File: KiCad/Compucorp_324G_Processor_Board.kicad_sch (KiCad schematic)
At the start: 9 parts, among them J5 Processor Interboard, J6 Test Connector, U5 TMC1872 (TCL07), U6 TMC1866 (TCL06), U7 TMC1867 (TCL05), U8 TMC1870 (TCL04)

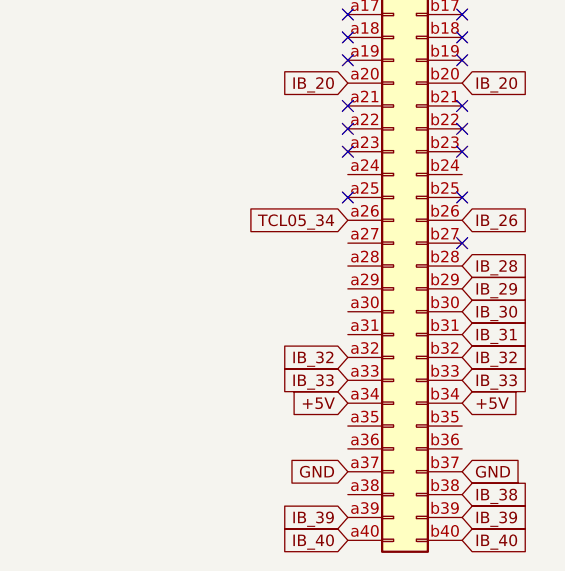
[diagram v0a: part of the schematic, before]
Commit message: Update Compucorp_324G_Processor_Board.kicad_sch
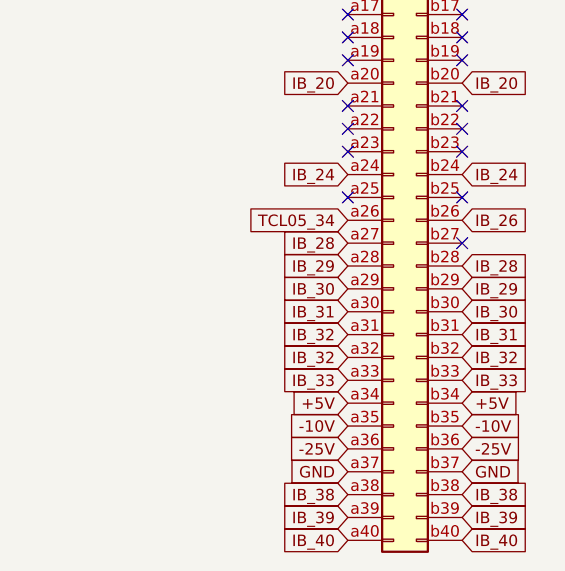
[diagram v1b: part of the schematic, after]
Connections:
- net IB_28: now also J5.a27 (Pin_a27)
- net IB_29: now also J5.a28 (Pin_a28)
- net IB_30: now also J5.a29 (Pin_a29)
- net IB_31: now also J5.a30 (Pin_a30)
- net IB_32: now also J5.a31 (Pin_a31)
- net IB_38: now also J5.a38 (Pin_a38)
- net IB_24: now reaches J5.a24 (Pin_a24)
- net IB_24: now also J5.b24 (Pin_b24)
- net -10V: now reaches J5.a35 (Pin_a35)
- net -10V: now also J5.b35 (Pin_b35)
- net -25V: now reaches J5.a36 (Pin_a36)
- net -25V: now also J5.b36 (Pin_b36)

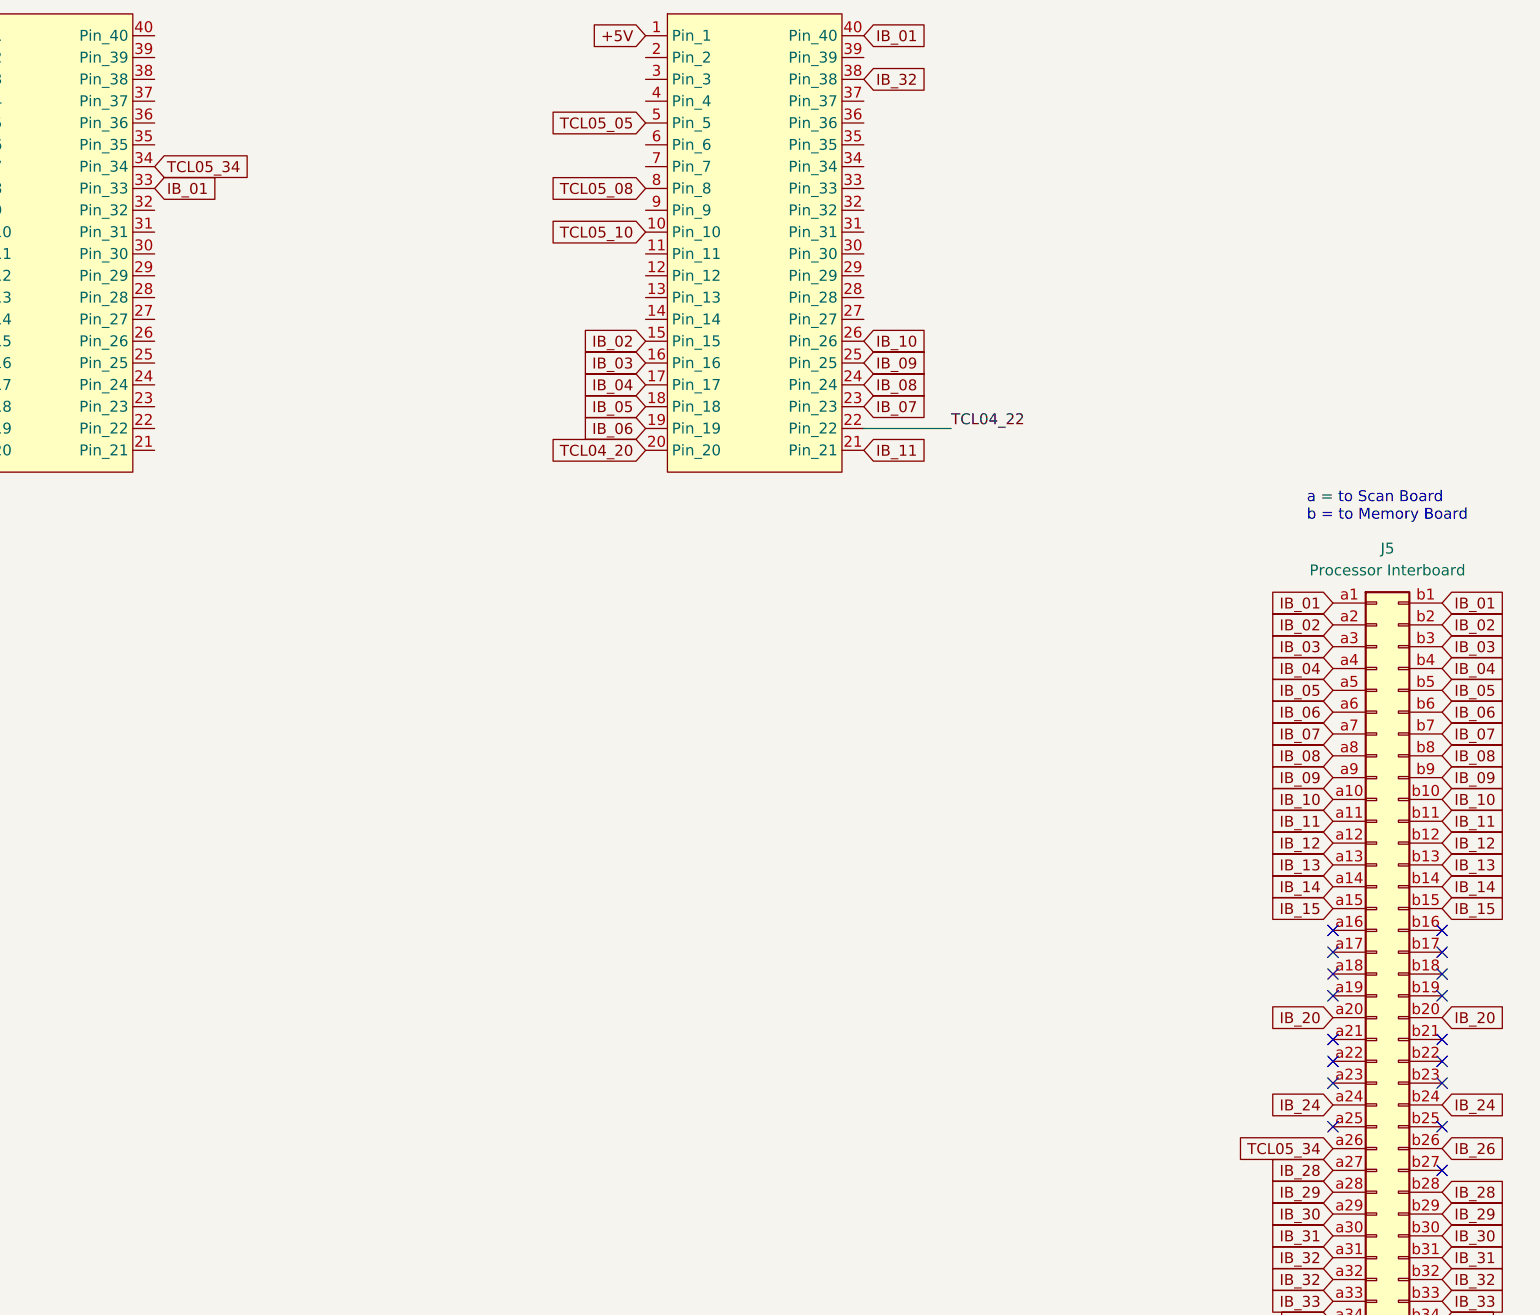
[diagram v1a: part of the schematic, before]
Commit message: Update Compucorp_324G_Processor_Board.kicad_sch
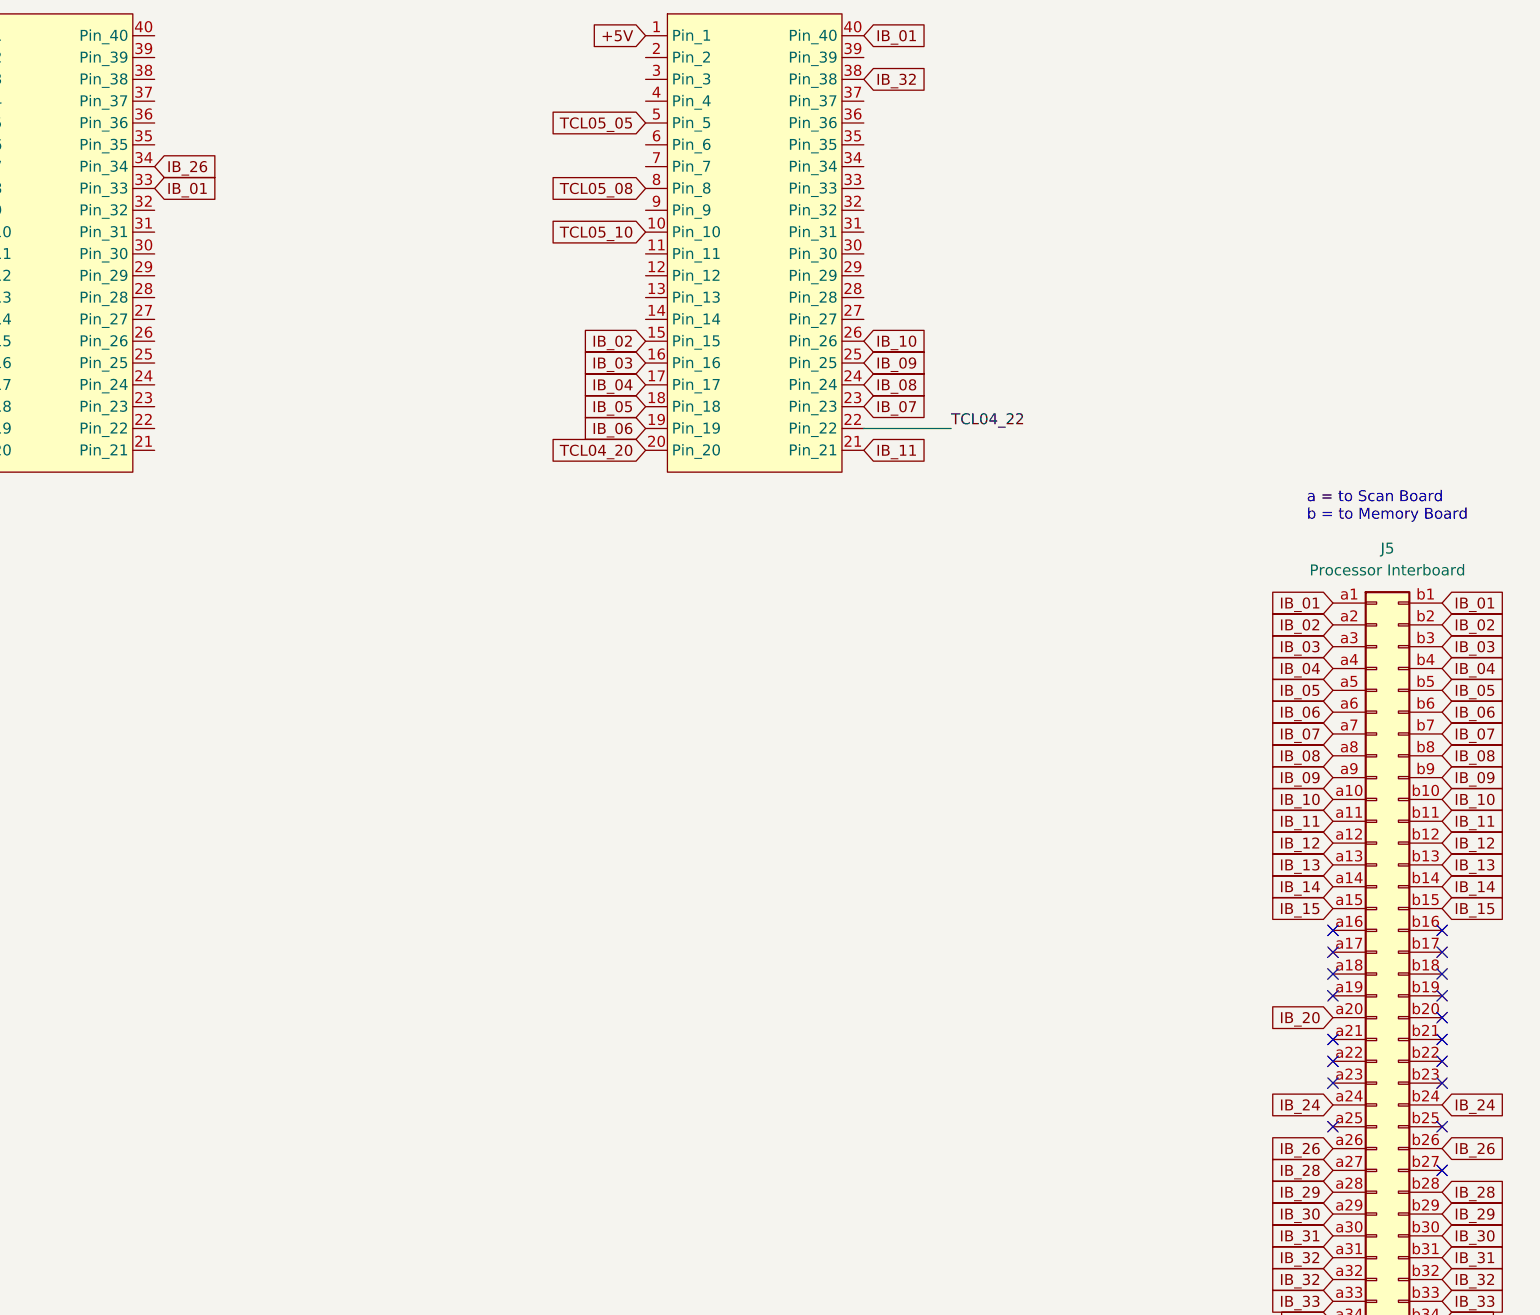
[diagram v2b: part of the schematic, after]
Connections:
- net TCL05_34 is gone; now on net IB_26: J5.a26 (Pin_a26), U7.34 (Pin_34)
- net IB_20: no longer J5.b20 (Pin_b20)
- no-connect marks 20 -> 21

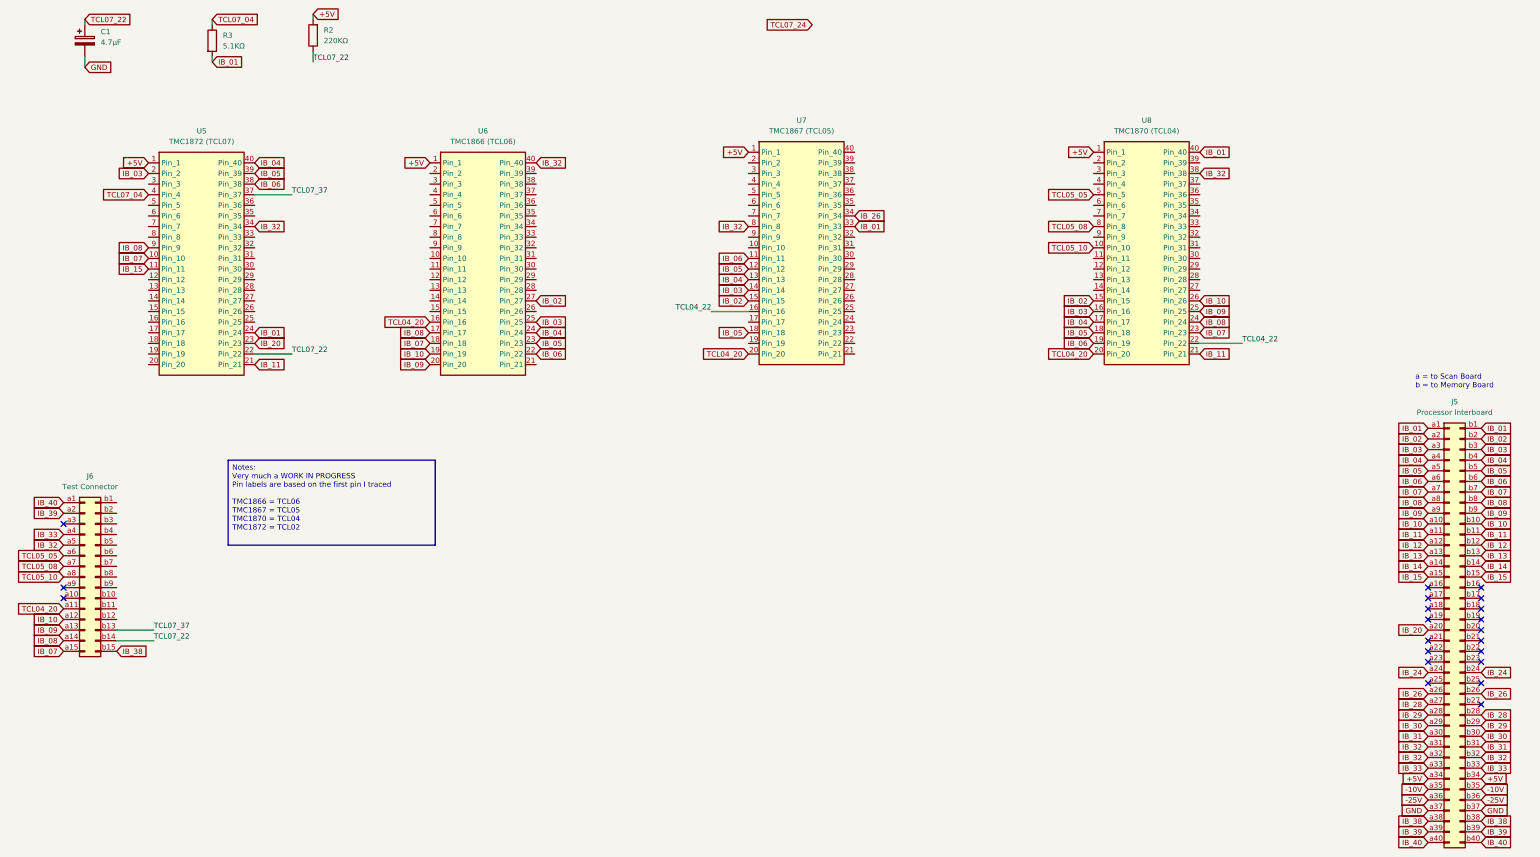
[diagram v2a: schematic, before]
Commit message: Update Compucorp_324G_Processor_Board.kicad_sch
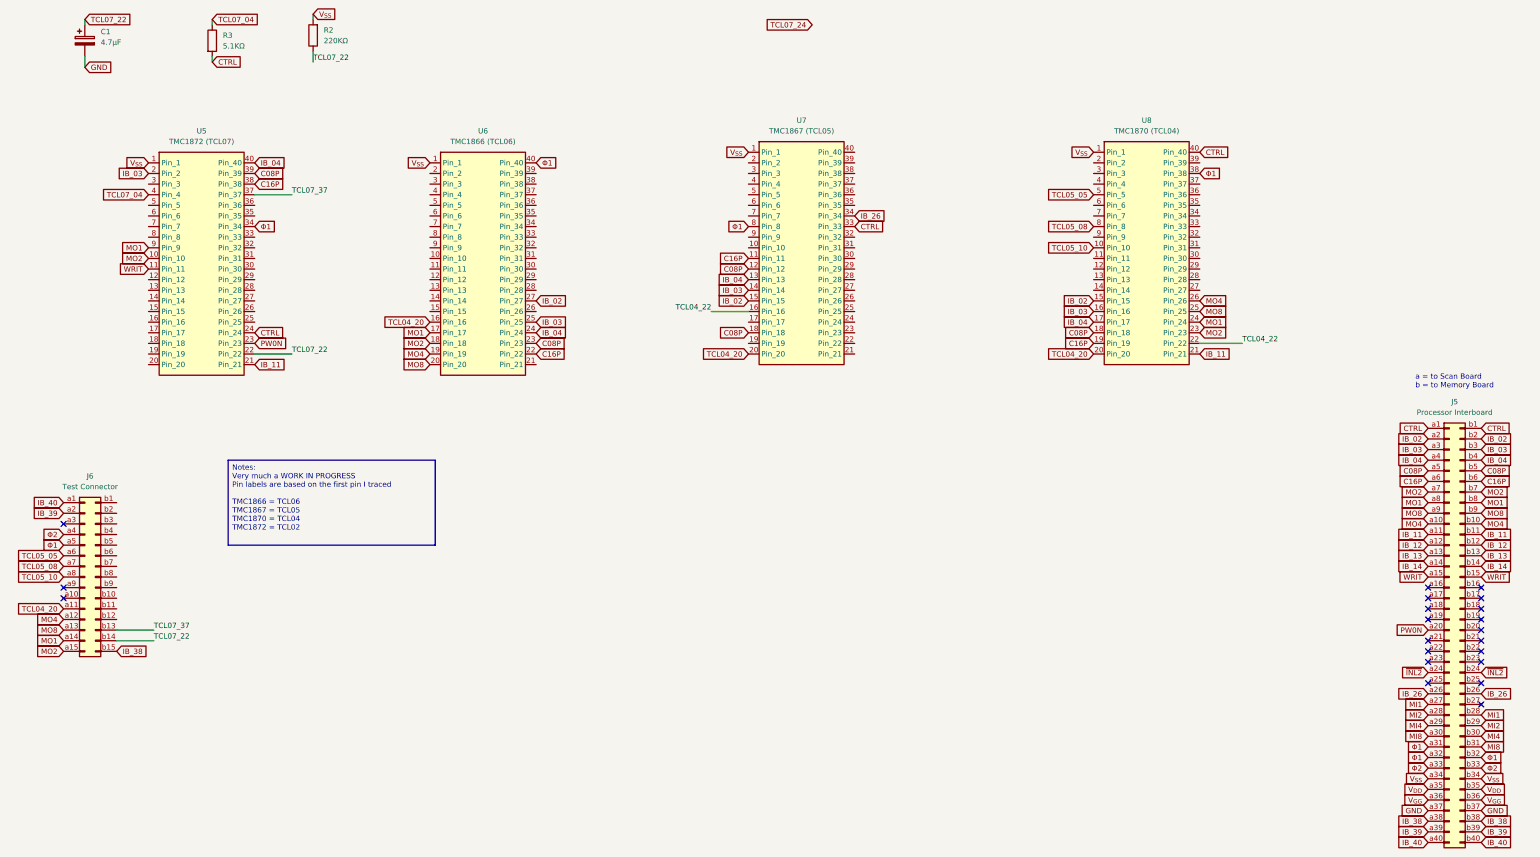
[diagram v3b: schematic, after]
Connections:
- net +5V renamed V_{SS}
- net -10V renamed V_{DD}
- net -25V renamed V_{GG}
- net IB_01 renamed CTRL
- net IB_05 renamed C08P
- net IB_06 renamed C16P
- net IB_07 renamed MO2
- net IB_08 renamed MO1
- net IB_09 renamed MO8
- net IB_10 renamed MO4
- net IB_15 renamed WRIT
- net IB_20 renamed PW0N
- net IB_24 renamed ~{INL2}
- net IB_28 renamed MI1
- net IB_29 renamed MI2
- net IB_30 renamed MI4
- net IB_31 renamed MI8
- net IB_32 renamed Φ1
- net IB_33 renamed Φ2
